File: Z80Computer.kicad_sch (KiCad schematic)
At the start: 12 parts, among them J1 Conn_Coaxial_Power, SW1 SW_Push, U1 Z80CPU, U2 28C256, U4 74LS138, U5 74LS00, U6 KM62256CLP, U7 74LS00, X1 CXO_DIP14

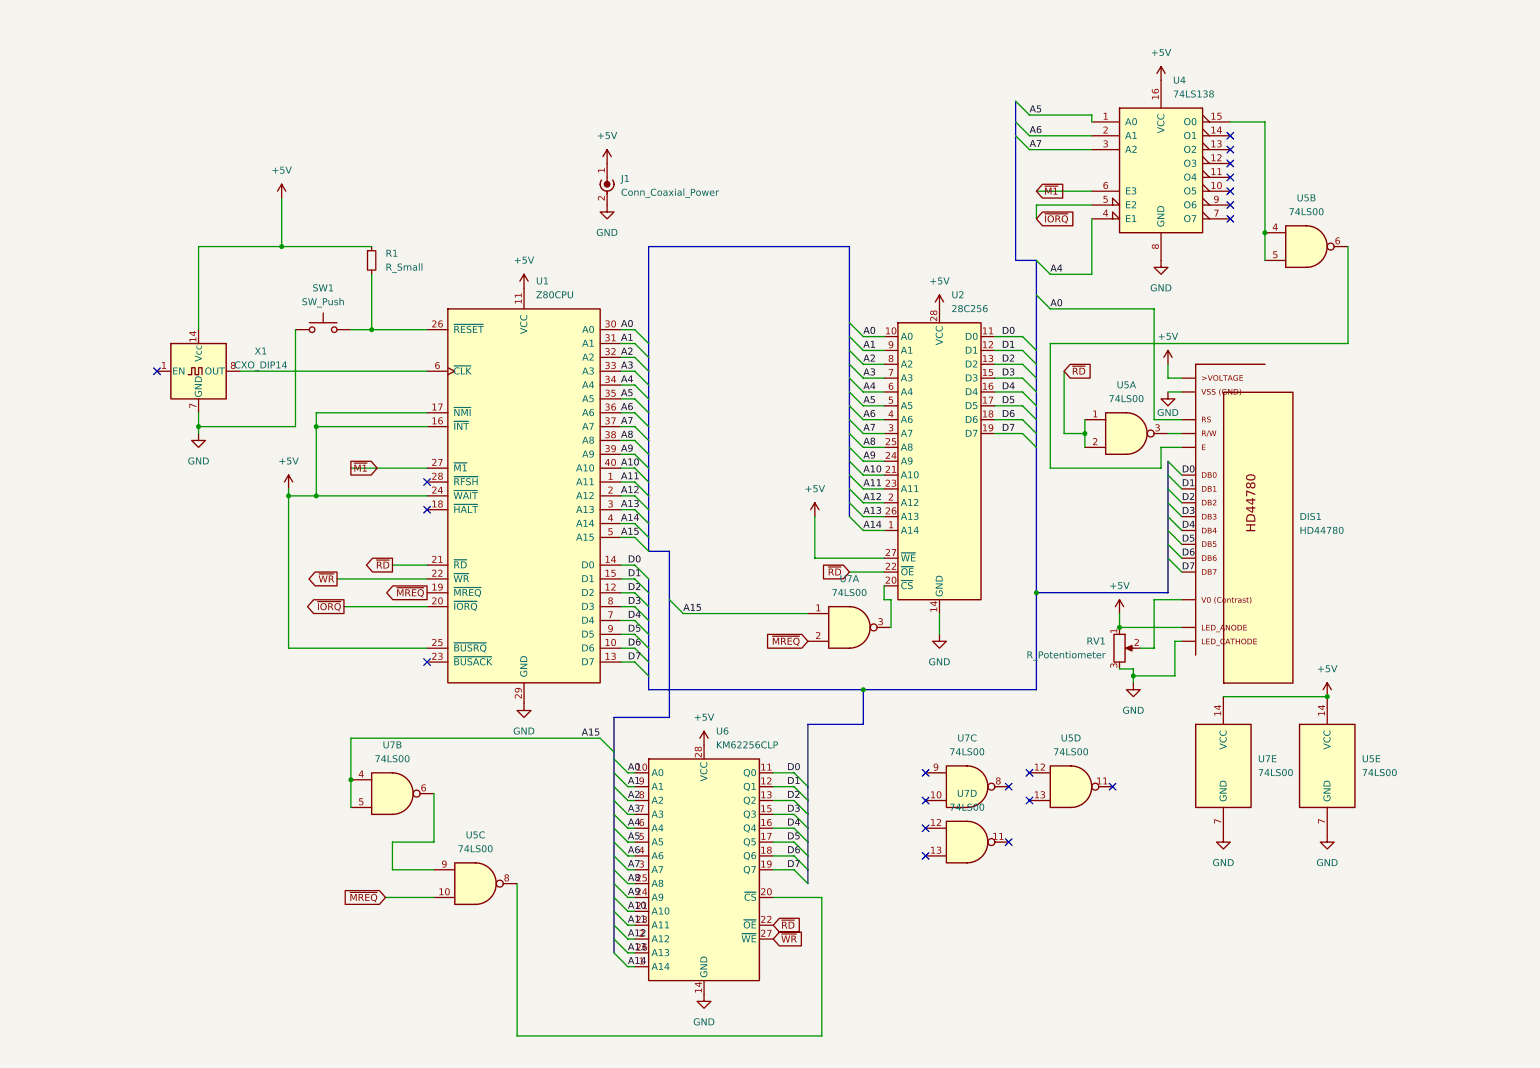
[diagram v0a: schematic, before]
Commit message: before auto route pcb
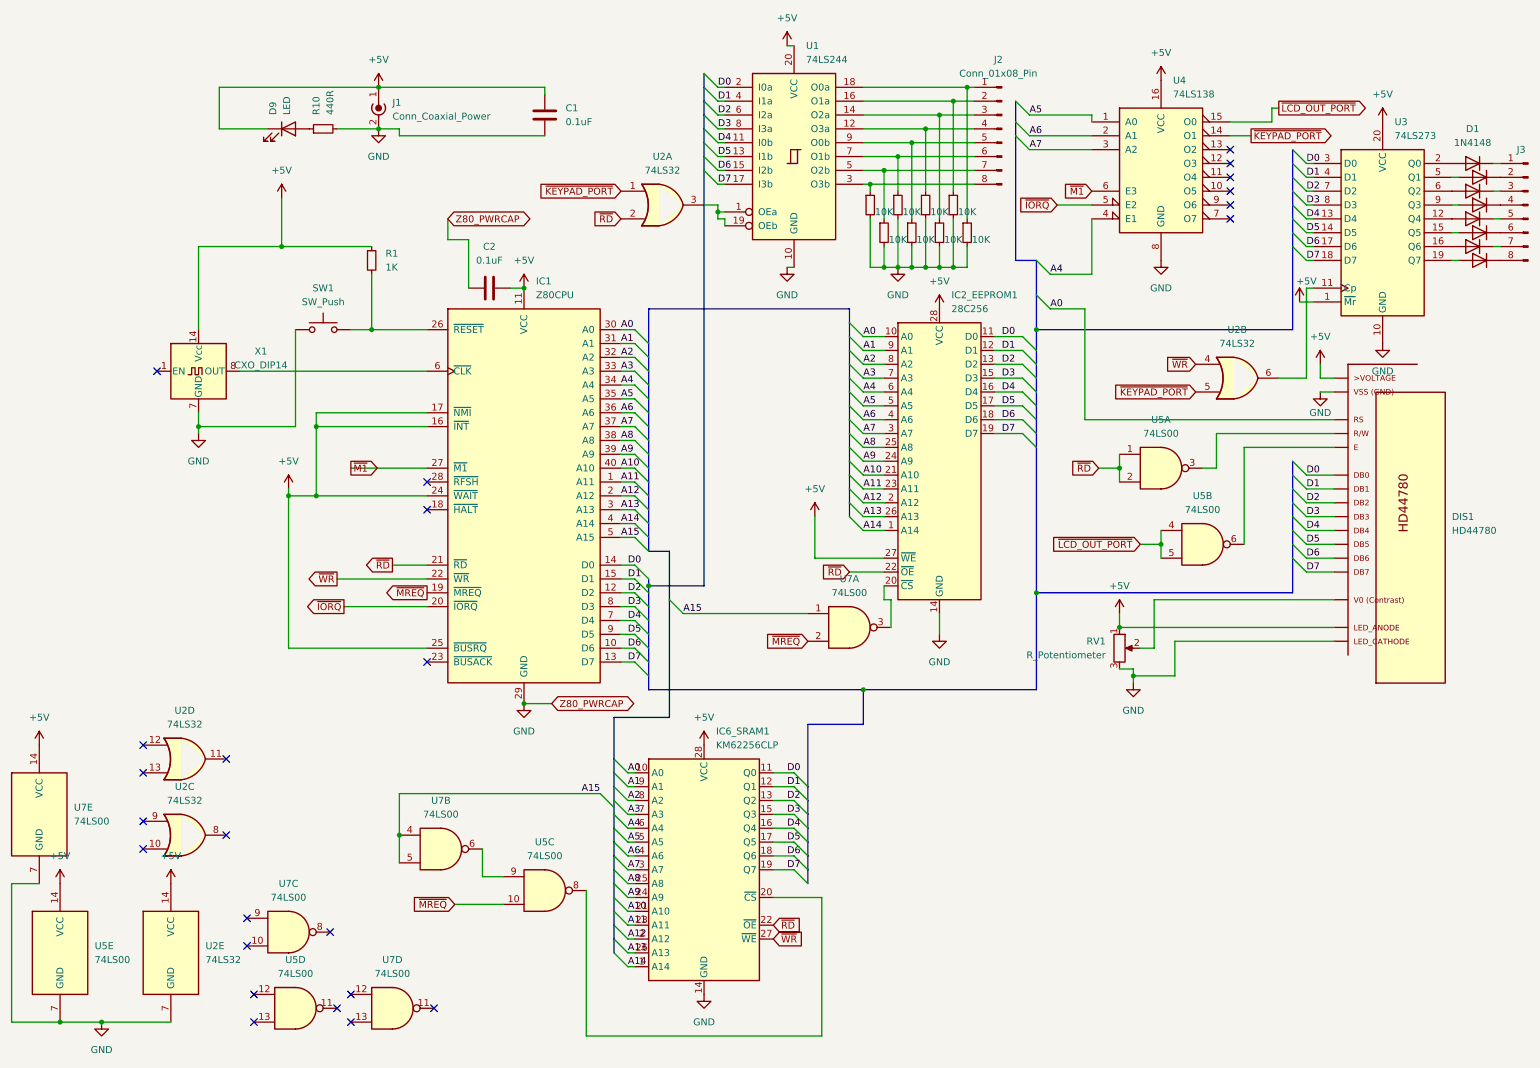
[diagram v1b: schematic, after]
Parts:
- added C1, C2: 0.1uF, Capacitor_THT:CP_Radial_D4.0mm_P1.50mm, symbol Z80ComputerLib:C
- added D1, D2, D3, D4, D5, D6, D7, D8: 1N4148, Diode_THT:D_DO-35_SOD27_P7.62mm_Horizontal, symbol Diode:1N4148
- added D9: LED, LED_THT:LED_D5.0mm, symbol Device:LED
- added J2, J3: Conn_01x08_Pin, Connector_JST:JST_EH_B8B-EH-A_1x08_P2.50mm_Vertical, symbol Connector:Conn_01x08_Pin
- added R10: 440R, Resistor_THT:R_Axial_DIN0204_L3.6mm_D1.6mm_P1.90mm_Vertical, symbol Z80ComputerLib:R_Small
- added R2, R3, R4, R5, R6, R7, R8, R9: 10K, Resistor_THT:R_Axial_DIN0204_L3.6mm_D1.6mm_P1.90mm_Vertical, symbol Z80ComputerLib:R_Small
- added U1: 74LS244, Package_DIP:DIP-20_W7.62mm, symbol Z80ComputerLib:74LS244
- added U2: 74LS32, Package_DIP:DIP-14_W7.62mm, symbol 74xx:74LS32
- added U3: 74LS273, Package_DIP:DIP-20_W7.62mm, symbol Z80ComputerLib:74LS273
- R1: value R_Small -> 1K
- U5, U7: footprint (none) -> Package_DIP:DIP-14_W7.62mm
- renumbered U1 to IC1, U2 to IC2_EEPROM1, U6 to IC6_SRAM1
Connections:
- net +5V: now also C1.1, C2.2, D9.1 (K), U1.20 (VCC), U2.14 (VCC), U3.1 (~{Mr}), U3.20 (VCC)
- net D0: now also U1.2 (I0a), U3.3 (D0)
- net D1: now also U1.4 (I1a), U3.4 (D1)
- net D2: now also U1.6 (I2a), U3.7 (D2)
- net D3: now also U1.8 (I3a), U3.8 (D3)
- net D4: now also U1.11 (I0b), U3.13 (D4)
- net D5: now also U1.13 (I1b), U3.14 (D5)
- net D6: now also U1.15 (I2b), U3.17 (D6)
- net D7: now also U1.17 (I3b), U3.18 (D7)
- net GND: now also C1.2, C2.1, R10.2, R2.2, R3.2, R4.2, R5.2, R6.2, R7.2, R8.2, R9.2, U1.10 (GND), U2.7 (GND), U3.10 (GND)
- net ~{RD}: now also U2.2
- net ~{WR}: now also U2.4
- net ~{KEYPAD_PORT}: now reaches U4.14 (O1)
- net ~{KEYPAD_PORT}: now also U2.1, U2.5
- net ~{LCD_OUT_PORT}: now reaches U4.15 (O0), U5.4, U5.5
- new net: J2.3 (Pin_3), R7.1, U1.14 (O2a)
- new net: J2.2 (Pin_2), R8.1, U1.16 (O1a)
- new net: J2.5 (Pin_5), R5.1, U1.9 (O0b)
- new net: D1.1 (K), J3.1 (Pin_1)
- new net: D8.1 (K), J3.2 (Pin_2)
- new net: D3.1 (K), J3.3 (Pin_3)
- new net: D2.1 (K), J3.4 (Pin_4)
- new net: D4.1 (K), J3.5 (Pin_5)
- new net: D6.1 (K), J3.6 (Pin_6)
- new net: D5.1 (K), J3.7 (Pin_7)
- new net: D7.1 (K), J3.8 (Pin_8)
- new net: D7.2 (A), U3.19 (Q7)
- new net: D6.2 (A), U3.15 (Q5)
- new net: D9.2 (A), R10.1
- new net: D1.2 (A), U3.2 (Q0)
- new net: D5.2 (A), U3.16 (Q6)
- new net: J2.8 (Pin_8), R2.1, U1.3 (O3b)
- new net: D8.2 (A), U3.5 (Q1)
- new net: J2.7 (Pin_7), R4.1, U1.5 (O2b)
- new net: U2.6, U3.11 (Cp)
- new net: D4.2 (A), U3.12 (Q4)
- new net: D3.2 (A), U3.6 (Q2)
- new net: D2.2 (A), U3.9 (Q3)
- new net: J2.1 (Pin_1), R9.1, U1.18 (O0a)
- new net: J2.4 (Pin_4), R6.1, U1.12 (O3a)
- new net: U1.1 (OEa), U1.19 (OEb), U2.3
- new net: J2.6 (Pin_6), R3.1, U1.7 (O1b)
- no-connect marks 20 -> 25
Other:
- title: (none) -> Minimal Z80 Computer
- moved on the sheet: DIS1, J1, U5A, U5B, U5C, U5D, U5E, U7B, U7C, U7D, U7E
